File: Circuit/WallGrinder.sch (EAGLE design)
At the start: 32 parts, among them IC2 MIC5225-5v, J5 1X04_SMD_STRAIGHT_COMBO, J6 1X04_SMD_STRAIGHT_COMBO

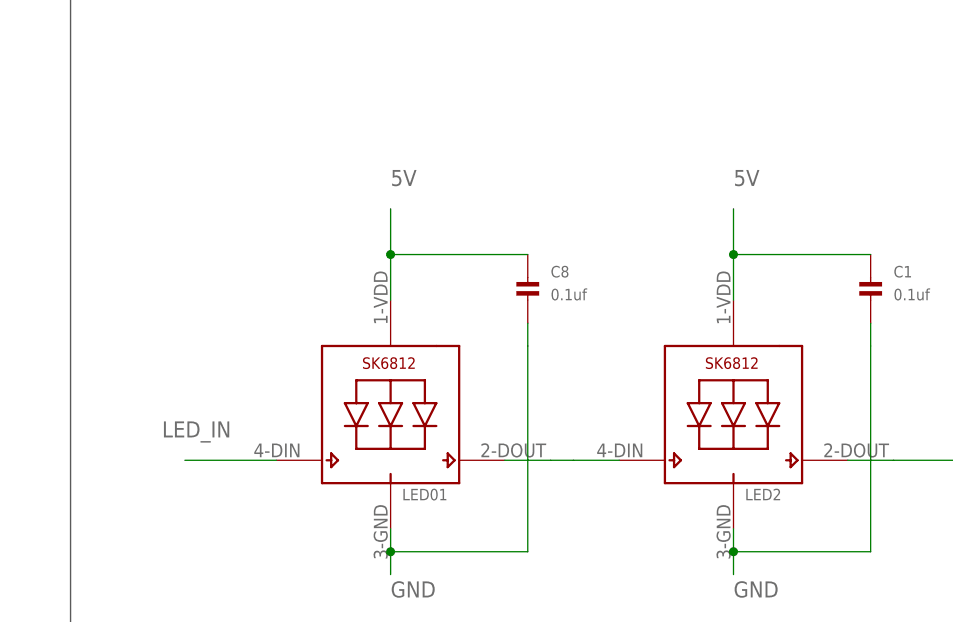
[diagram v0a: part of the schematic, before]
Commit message: movement
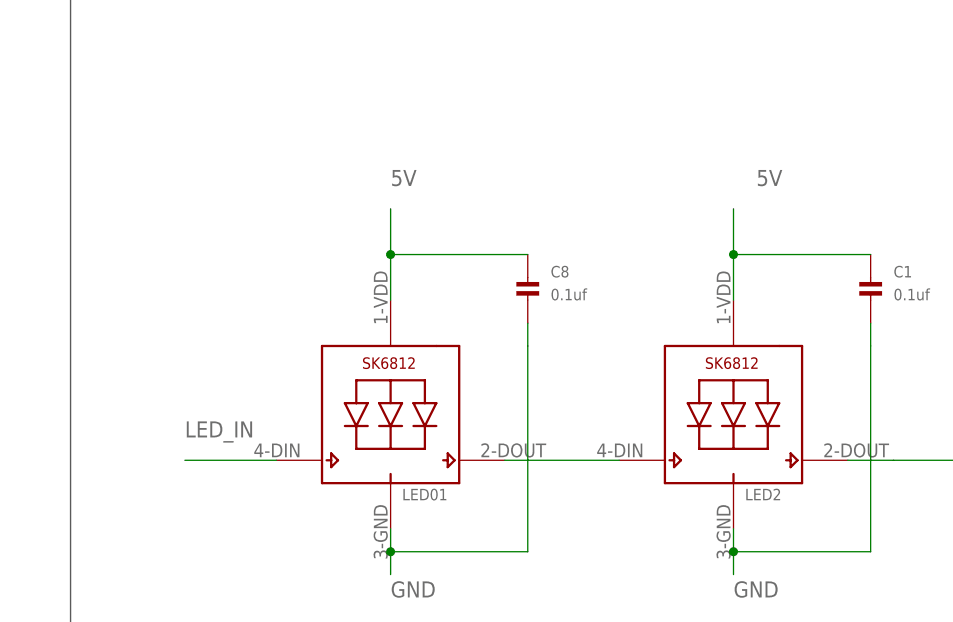
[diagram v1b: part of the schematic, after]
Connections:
- new net N$3: LED01.DO, LED2.DI
- net LED_IN: no longer LED01.DO, LED2.DI
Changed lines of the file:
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@@
 </variantdefs>
 <classes>
-<class number="0" name="default" width="0" drill="0">
+<class number="0" name="default" width="0.22" drill="0">
+<clearance class="0" value="0.225"/>
 </class>
 </classes>
@@
 <net name="LED_IN" class="0">
 <segment>
-<pinref part="LED01" gate="G$1" pin="DI"/>
-<wire x1="386.08" y1="299.72" x2="375.92" y2="299.72" width="0.1524" layer="91"/>
-<label x="373.38" y="302.26" size="1.778" layer="95"/>
-</segment>
-<segment>
 <pinref part="U$5" gate="G$1" pin="16/A2/T"/>
 <wire x1="426.72" y1="419.1" x2="421.64" y2="419.1" width="0.1524" layer="91"/>
@@
 </segment>
 <segment>
-<pinref part="LED2" gate="G$1" pin="DI"/>
-<wire x1="424.18" y1="299.72" x2="419.1" y2="299.72" width="0.1524" layer="91"/>
-<pinref part="LED01" gate="G$1" pin="DO"/>
-<wire x1="411.48" y1="299.72" x2="416.56" y2="299.72" width="0.1524" layer="91"/>
-<wire x1="416.56" y1="299.72" x2="419.1" y2="299.72" width="0.1524" layer="91"/>
+<pinref part="LED01" gate="G$1" pin="DI"/>
+<wire x1="386.08" y1="299.72" x2="375.92" y2="299.72" width="0.1524" layer="91"/>
+<label x="375.92" y="302.26" size="1.778" layer="95"/>
 </segment>
 </net>
@@
 <junction x="436.88" y="322.58"/>
 <pinref part="C1" gate="G$1" pin="P$1"/>
-<label x="436.88" y="330.2" size="1.778" layer="95"/>
+<label x="439.42" y="330.2" size="1.778" layer="95"/>
 </segment>
 <segment>
@@
 </segment>
 </net>
+<net name="N$3" class="0">
+<segment>
+<pinref part="LED01" gate="G$1" pin="DO"/>
+<pinref part="LED2" gate="G$1" pin="DI"/>
+<wire x1="411.48" y1="299.72" x2="424.18" y2="299.72" width="0.1524" layer="91"/>
+</segment>
+</net>
